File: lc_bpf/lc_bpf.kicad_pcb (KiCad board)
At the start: 2 copper layers, 47 x 47 mm, 27 parts, among them J2 Conn_01x03, J3 Conn_01x03

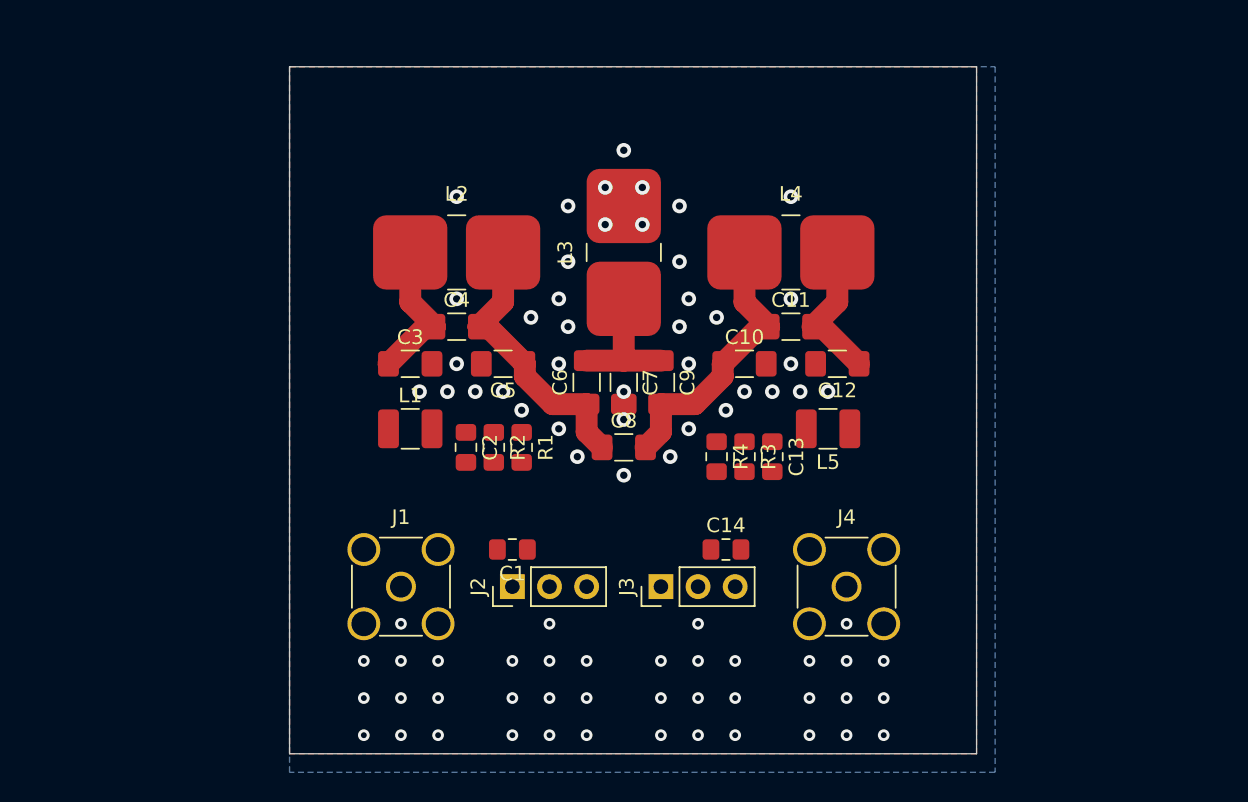
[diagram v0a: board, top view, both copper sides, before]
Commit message: Change filter layout
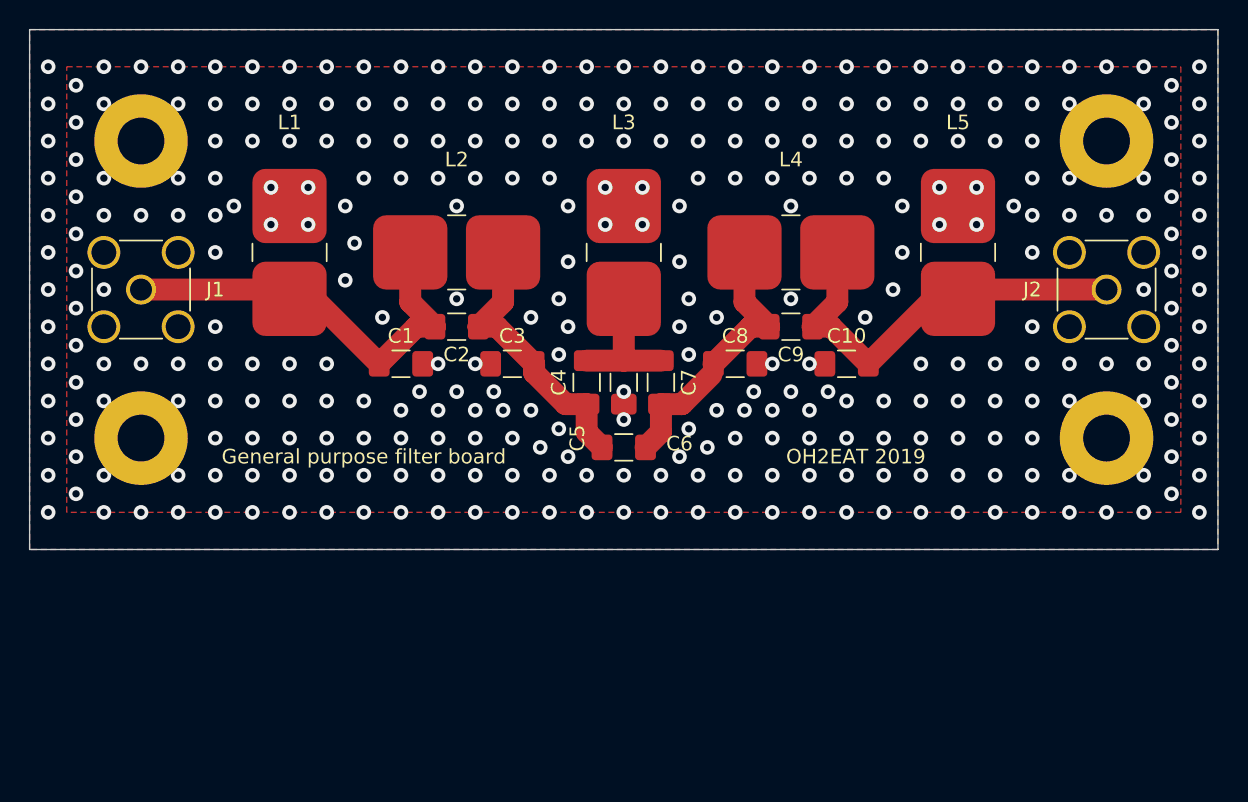
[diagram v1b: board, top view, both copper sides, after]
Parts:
- removed C13, C14: C, Capacitor_SMD:C_0805_2012Metric_Pad1.15x1.40mm_HandSolder
- removed the C2 at (62.9, 76.8)
- removed the C3 at (59.1, 71.1)
- removed the J2 at (66.0, 86.4)
- removed J3: Conn_01x03, Connector_PinHeader_2.54mm:PinHeader_1x03_P2.54mm_Vertical
- removed R1, R2, R3, R4: R, Resistor_SMD:R_0805_2012Metric_Pad1.15x1.40mm_HandSolder
- added H1: ~, MountingHole:MountingHole_3.2mm_M3_Pad, F.Cu at (40.6, 55.9)
- added H2: ~, MountingHole:MountingHole_3.2mm_M3_Pad, F.Cu at (40.6, 76.2)
- added H3: ~, MountingHole:MountingHole_3.2mm_M3_Pad, F.Cu at (106.7, 55.9)
- added H4: ~, MountingHole:MountingHole_3.2mm_M3_Pad, F.Cu at (106.7, 76.2)
- C1: footprint Capacitor_SMD:C_0805_2012Metric_Pad1.15x1.40mm_HandSolder -> Capacitor_SMD:C_1206_3216Metric_Pad1.42x1.75mm_HandSolder
- L1, L5: footprint Inductor_SMD:L_1210_3225Metric_Pad1.42x2.65mm_HandSolder -> lc_bpf:L
- moved J1 27.0 mm to (40.6, 66.0)
- moved J2 27.0 mm to (106.7, 66.0)
- moved L5 15.0 mm to (96.5, 63.5), turned to 90 degrees
- moved C1 14.8 mm to (58.4, 71.1), turned to 0 degrees
- moved L1 14.6 mm to (50.8, 63.5), turned to 90 degrees
- moved C10 0.64 mm to (88.9, 71.1)
- moved C3 0.64 mm to (66.0, 71.1)
- moved C8 0.64 mm to (81.3, 71.1)
- renumbered C12 to C10, C4 to C2, C5 to C3, C6 to C4, C7 to C5, C8 to C6, C9 to C7, C10 to C8, C11 to C9, J4 to J2
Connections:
- C2 pad 1: Net-(C3-Pad1) -> Net-(C1-Pad1)
- J1 pad 1: Net-(C3-Pad1) -> Net-(C1-Pad1)
- L1 pad 1: Net-(C3-Pad1) -> Net-(C1-Pad1)
- L1 pad 2: Net-(C2-Pad1) -> GND
- L2 pad 1: Net-(C3-Pad1) -> Net-(C1-Pad1)
- L5 pad 2: Net-(C13-Pad1) -> GND
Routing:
- net Net-(C1-Pad1): track 0.00 -> 29.0 mm
- net Net-(C10-Pad1): track 10.0 -> 29.0 mm
- net Net-(C3-Pad1): track 10.0 -> 0.00 mm
- net Net-(C6-Pad2): track 19.3 -> 18.3 mm
- net GND: vias 80 -> 329
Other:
- board size 47 x 47 mm -> 81.3 x 35.6 mm
- board text added: "General purpose filter board"
- board text added: "OH2EAT 2019"
